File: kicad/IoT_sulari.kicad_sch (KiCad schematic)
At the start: 37 parts, among them J1 73412-0110, J2 73412-0110, J3 20021121-00010C4LF, J4 20021121-00010C4LF, J6 20021121-00010C4LF, SW1 SW_SPST, SW2 TL3301DF160QG, SW3 TL3301DF160QG, SW4 TL3301DF160QG, SW5 TL3301DF160QG, U2 NRF9160

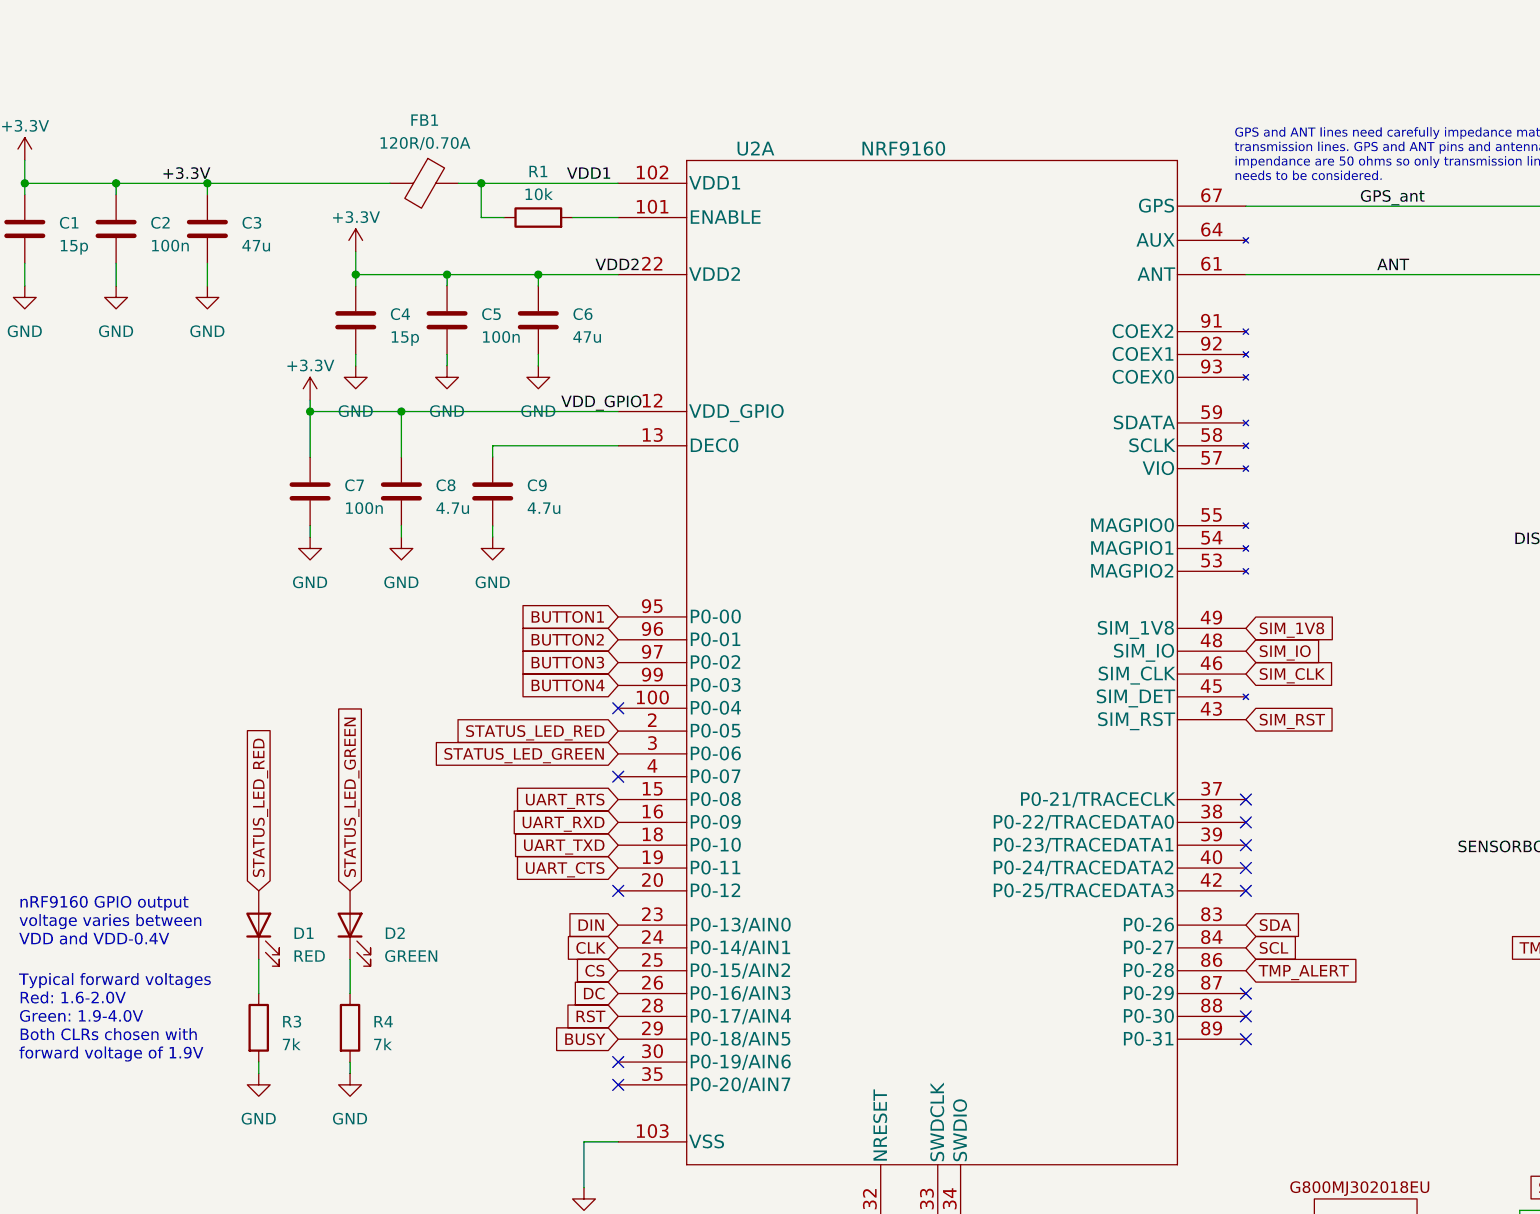
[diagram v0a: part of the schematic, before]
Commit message: routing
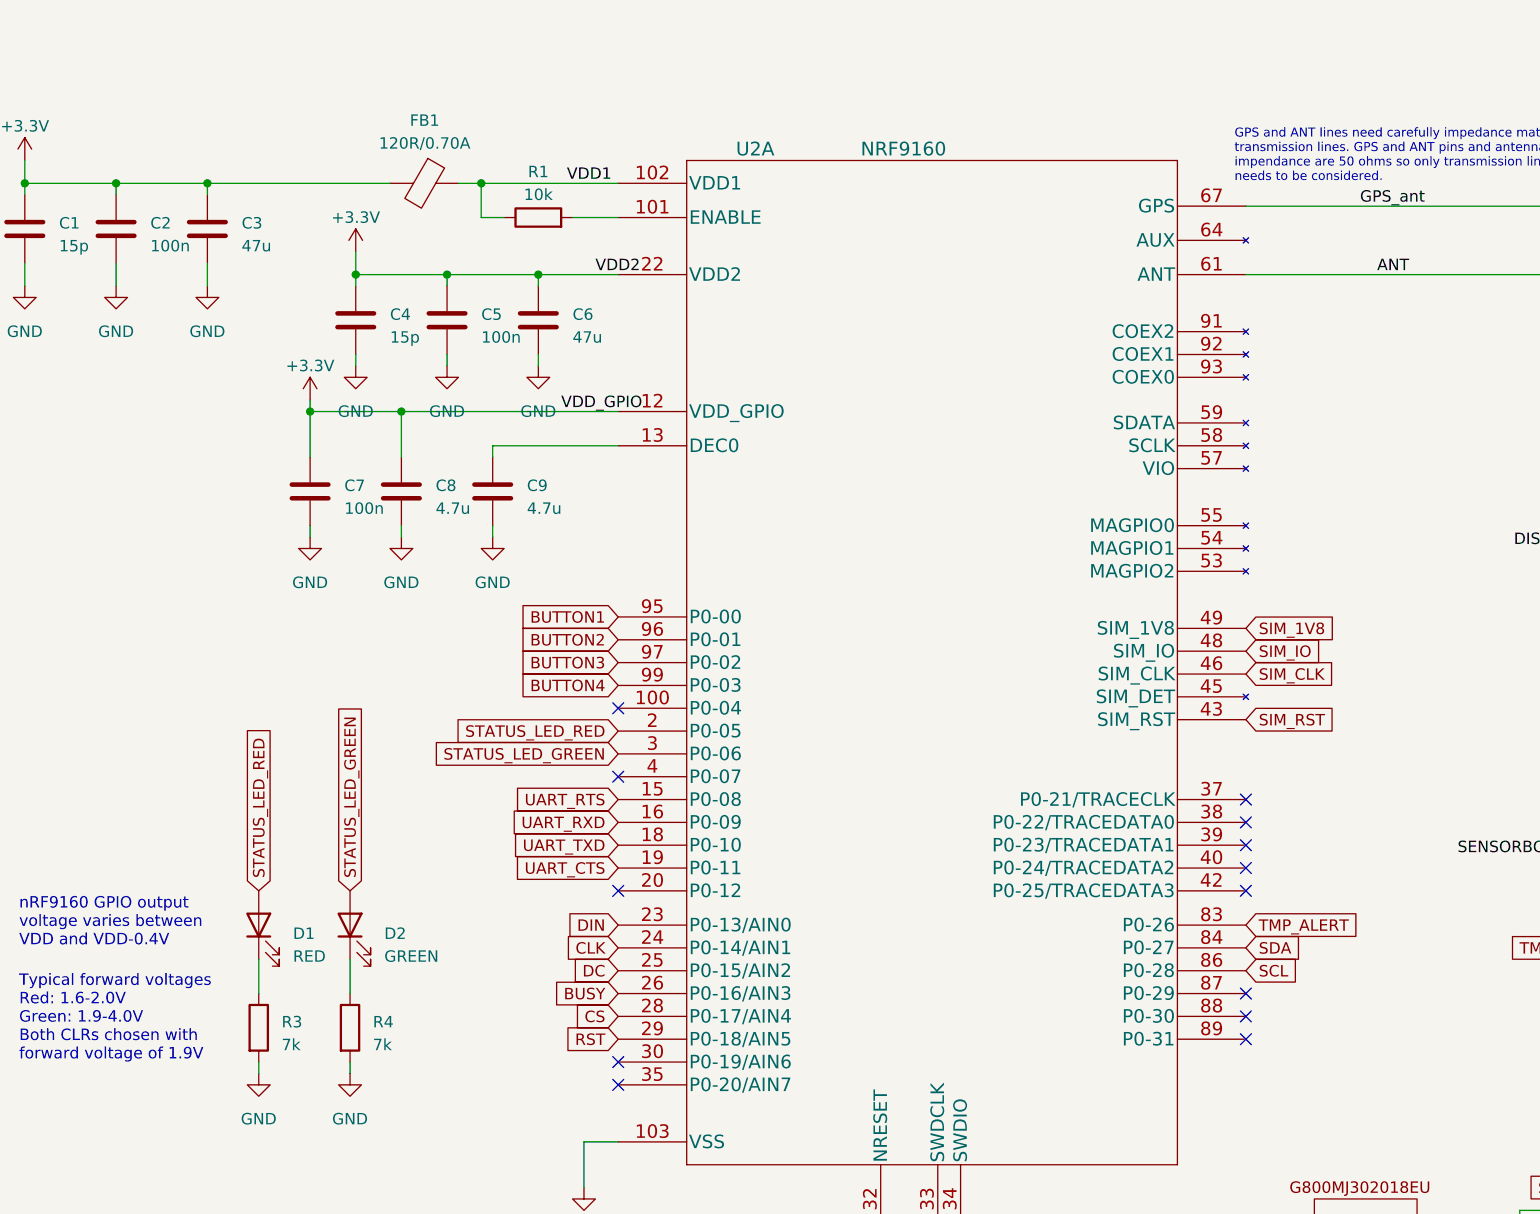
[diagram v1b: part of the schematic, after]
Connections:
- net BUSY: now also U2.26 (P0-16/AIN3); no longer U2.29 (P0-18/AIN5)
- net CS: now also U2.28 (P0-17/AIN4); no longer U2.25 (P0-15/AIN2)
- net DC: now also U2.25 (P0-15/AIN2); no longer U2.26 (P0-16/AIN3)
- net RST: now also U2.29 (P0-18/AIN5); no longer U2.28 (P0-17/AIN4)
- net SCL: now also U2.86 (P0-28); no longer U2.84 (P0-27)
- net SDA: now also U2.84 (P0-27); no longer U2.83 (P0-26)
- net TMP_ALERT: now also U2.83 (P0-26); no longer U2.86 (P0-28)
- net +3.3V: no longer names the net of C1.1, C2.1, C3.1, FB1.2
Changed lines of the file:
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@@
-    (effects (font (size 1.27 1.27)) (justify left bottom))
-  )
-  (label "+3.3V" (at 101.6 24.13 0) (fields_autoplaced)
     (effects (font (size 1.27 1.27)) (justify left bottom))
   )
@@
     )
   )
-  (global_label "TMP_ALERT" (shape input) (at 222.25 111.76 0) (fields_autoplaced)
+  (global_label "TMP_ALERT" (shape input) (at 222.25 106.68 0) (fields_autoplaced)
     (effects (font (size 1.27 1.27)) (justify left))
-    (property "Intersheetrefs" "${INTERSHEET_REFS}" (at 235.3157 111.76 0)
+    (property "Intersheetrefs" "${INTERSHEET_REFS}" (at 235.3157 106.68 0)
       (effects (font (size 1.27 1.27)) (justify left) hide)
     )
   )
-  (global_label "BUSY" (shape input) (at 152.4 119.38 180) (fields_autoplaced)
-    (effects (font (size 1.27 1.27)) (justify right))
-    (property "Intersheetrefs" "${INTERSHEET_REFS}" (at 144.5956 119.38 0)
+  (global_label "BUSY" (shape input) (at 152.4 114.3 180) (fields_autoplaced)
+    (effects (font (size 1.27 1.27)) (justify right))
+    (property "Intersheetrefs" "${INTERSHEET_REFS}" (at 144.5956 114.3 0)
       (effects (font (size 1.27 1.27)) (justify right) hide)
     )
@@
     )
   )
-  (global_label "RST" (shape input) (at 152.4 116.84 180) (fields_autoplaced)
-    (effects (font (size 1.27 1.27)) (justify right))
-    (property "Intersheetrefs" "${INTERSHEET_REFS}" (at 146.0471 116.84 0)
+  (global_label "RST" (shape input) (at 152.4 119.38 180) (fields_autoplaced)
+    (effects (font (size 1.27 1.27)) (justify right))
+    (property "Intersheetrefs" "${INTERSHEET_REFS}" (at 146.0471 119.38 0)
       (effects (font (size 1.27 1.27)) (justify right) hide)
     )
@@
     )
   )
-  (global_label "CS" (shape input) (at 152.4 111.76 180) (fields_autoplaced)
-    (effects (font (size 1.27 1.27)) (justify right))
-    (property "Intersheetrefs" "${INTERSHEET_REFS}" (at 147.0147 111.76 0)
+  (global_label "CS" (shape input) (at 152.4 116.84 180) (fields_autoplaced)
+    (effects (font (size 1.27 1.27)) (justify right))
+    (property "Intersheetrefs" "${INTERSHEET_REFS}" (at 147.0147 116.84 0)
       (effects (font (size 1.27 1.27)) (justify right) hide)
     )
@@
     )
   )
-  (global_label "SCL" (shape input) (at 222.25 109.22 0) (fields_autoplaced)
+  (global_label "SCL" (shape input) (at 222.25 111.76 0) (fields_autoplaced)
     (effects (font (size 1.27 1.27)) (justify left))
-    (property "Intersheetrefs" "${INTERSHEET_REFS}" (at 228.6634 109.22 0)
+    (property "Intersheetrefs" "${INTERSHEET_REFS}" (at 228.6634 111.76 0)
       (effects (font (size 1.27 1.27)) (justify left) hide)
     )
@@
     )
   )
-  (global_label "DC" (shape input) (at 152.4 114.3 180) (fields_autoplaced)
-    (effects (font (size 1.27 1.27)) (justify right))
-    (property "Intersheetrefs" "${INTERSHEET_REFS}" (at 146.9542 114.3 0)
+  (global_label "DC" (shape input) (at 152.4 111.76 180) (fields_autoplaced)
+    (effects (font (size 1.27 1.27)) (justify right))
+    (property "Intersheetrefs" "${INTERSHEET_REFS}" (at 146.9542 111.76 0)
       (effects (font (size 1.27 1.27)) (justify right) hide)
     )
@@
     )
   )
-  (global_label "SDA" (shape input) (at 222.25 106.68 0) (fields_autoplaced)
+  (global_label "SDA" (shape input) (at 222.25 109.22 0) (fields_autoplaced)
     (effects (font (size 1.27 1.27)) (justify left))
-    (property "Intersheetrefs" "${INTERSHEET_REFS}" (at 228.7239 106.68 0)
+    (property "Intersheetrefs" "${INTERSHEET_REFS}" (at 228.7239 109.22 0)
       (effects (font (size 1.27 1.27)) (justify left) hide)
     )
@@
   (symbol (lib_name "+3.3V_2") (lib_id "power:+3.3V") (at 86.36 21.59 0) (unit 1)
     (in_bom yes) (on_board yes) (dnp no) (fields_autoplaced)
-    (property "Reference" "#PWR011" (at 86.36 25.4 0)
+    (property "Reference" "#PWR0106" (at 86.36 25.4 0)
       (effects (font (size 1.27 1.27)) hide)
     )
@@
       (project "IoT_sulari"
         (path "/184b47ed-2c2b-4c02-be35-d18f4f4e5685"
-          (reference "#PWR011") (unit 1)
+          (reference "#PWR0106") (unit 1)
         )
       )
@@
   (symbol (lib_name "+3.3V_1") (lib_id "power:+3.3V") (at 123.19 31.75 0) (unit 1)
     (in_bom yes) (on_board yes) (dnp no) (fields_autoplaced)
-    (property "Reference" "#PWR012" (at 123.19 35.56 0)
+    (property "Reference" "#PWR0104" (at 123.19 35.56 0)
       (effects (font (size 1.27 1.27)) hide)
     )
@@
       (project "IoT_sulari"
         (path "/184b47ed-2c2b-4c02-be35-d18f4f4e5685"
-          (reference "#PWR012") (unit 1)
+          (reference "#PWR0104") (unit 1)
         )
       )
@@
   (symbol (lib_name "+3.3V_3") (lib_id "power:+3.3V") (at 118.11 48.26 0) (unit 1)
     (in_bom yes) (on_board yes) (dnp no) (fields_autoplaced)
-    (property "Reference" "#PWR025" (at 118.11 52.07 0)
+    (property "Reference" "#PWR0105" (at 118.11 52.07 0)
       (effects (font (size 1.27 1.27)) hide)
     )
@@
       (project "IoT_sulari"
         (path "/184b47ed-2c2b-4c02-be35-d18f4f4e5685"
-          (reference "#PWR025") (unit 1)
-        )
-      )
+          (reference "#PWR0105") (unit 1)
+        )
+      )
